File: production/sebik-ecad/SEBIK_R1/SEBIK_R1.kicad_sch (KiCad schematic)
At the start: 87 parts, among them J1 Conn_01x06_Male, J10 Conn_01x02_Male, J11 Conn_01x03_Male, J11 USB_B, J12 Conn_01x02_Male, J13 Conn_01x02_Male, J2 Conn_01x02_Male, J3 Conn_01x02_Male, J4 Conn_01x02_Male, J5 Conn_01x02_Male, J6 Conn_01x02_Male, J7 Conn_01x03_Male, J8 Conn_01x01_Male, J9 Conn_01x01_Male, Q1 2N7002, Q2 2N7002, Q3 2N7002, U1 ATmega328-A, U2 MCP23017_SO, U3 USBLC6-2SC6, U4 FT232RL, U5 MAX31855EASA, U6 MAX31855EASA, U7 MAX31855EASA, U8 LP2985-5.0, Y1 16Mhz

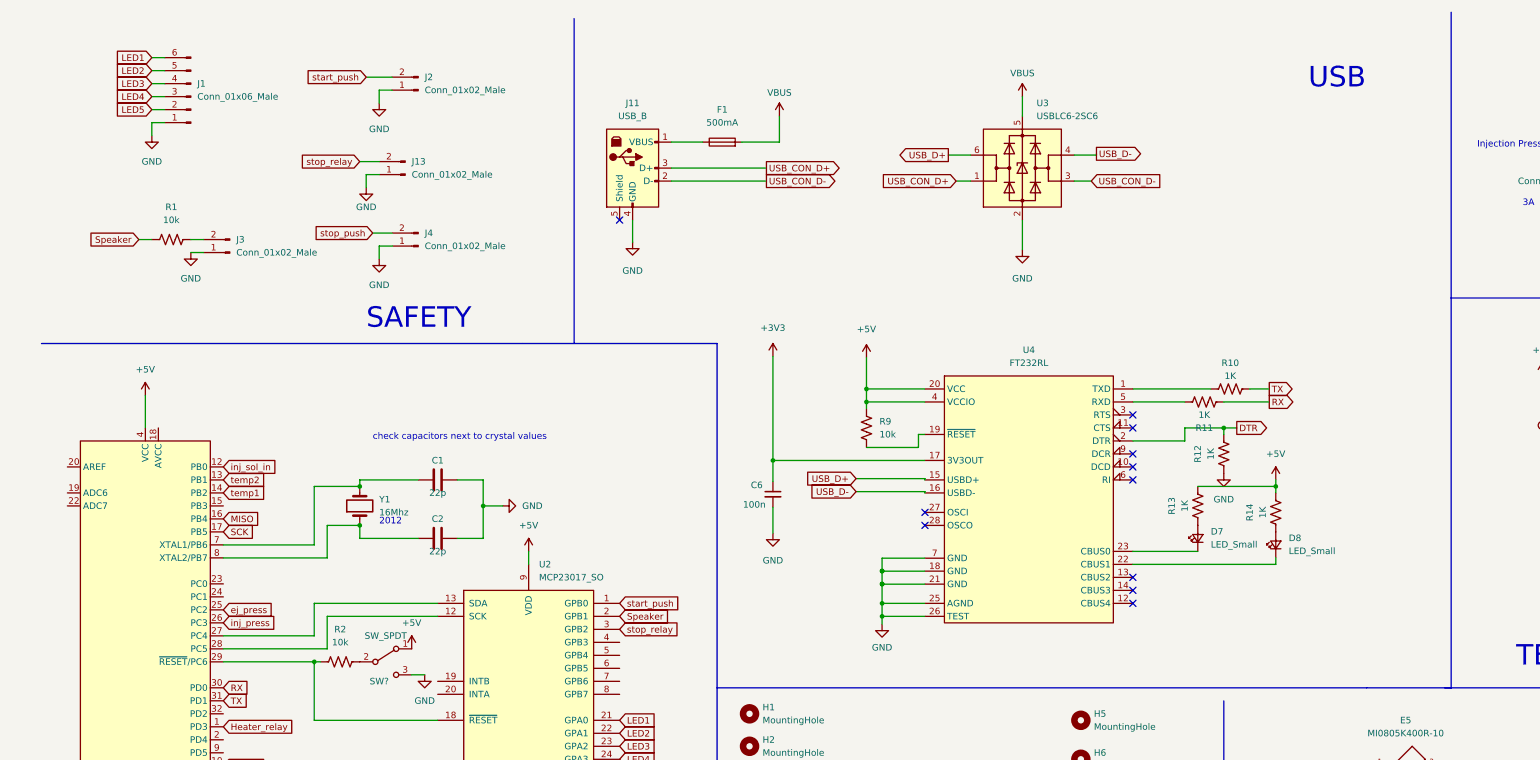
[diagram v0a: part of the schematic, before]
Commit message: Addressed comments from Nick
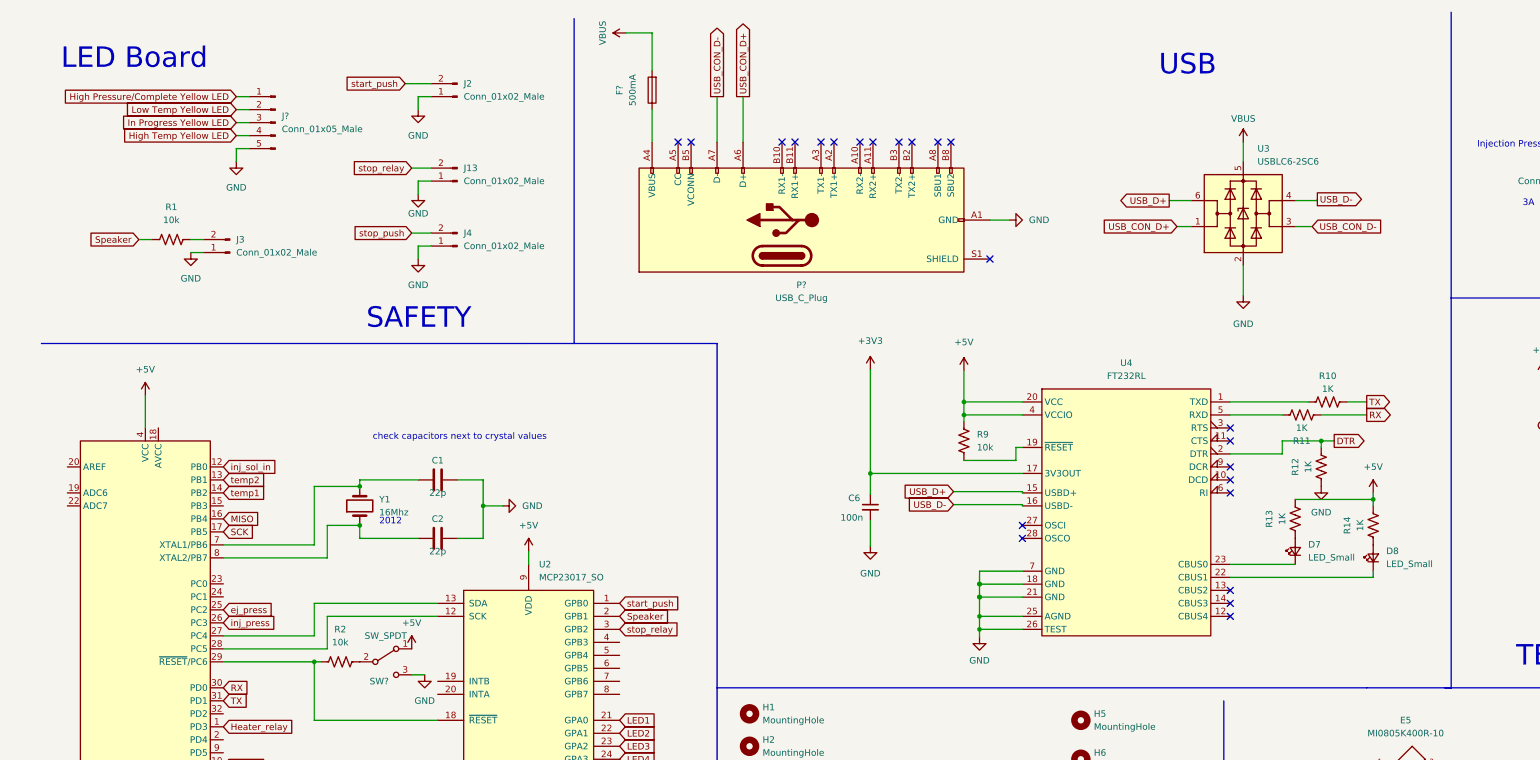
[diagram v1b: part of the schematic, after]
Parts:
- removed F1: 500mA, Fuse:Fuse_1210_3225Metric, symbol Device:Fuse
- removed J1: Conn_01x06_Male, Connector_JST:JST_XH_B6B-XH-AM_1x06_P2.50mm_Vertical, symbol Connector:Conn_01x06_Male
- removed J11: USB_B, Connector_USB:USB_Micro-B_Amphenol_10104110_Horizontal, symbol Connector:USB_B
- added F?: 500mA, Fuse:Fuse_1210_3225Metric, symbol Device:Fuse
- added J?: Conn_01x05_Male, symbol Connector:Conn_01x05_Male
- added P?: USB_C_Plug, symbol Connector:USB_C_Plug
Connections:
- net GND: now also J?.5 (Pin_5), P?.A1 (GND), P?.A12 (GND), P?.B1 (GND), P?.B12 (GND)
- net USB_CON_D+: now also P?.A6 (D+)
- net USB_CON_D-: now also P?.A7 (D-)
- net VBUS: now also F?.2
- new net: F?.1, P?.A4 (VBUS), P?.A9 (VBUS), P?.B4 (VBUS), P?.B9 (VBUS)
- new net High Pressure/Complete Yellow LED: J?.1 (Pin_1)
- new net High Temp Yellow LED: J?.4 (Pin_4)
- new net In Progress Yellow LED: J?.3 (Pin_3)
- new net Low Temp Yellow LED: J?.2 (Pin_2)
- no-connect marks 11 -> 23
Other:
- note added: "LED Board"
- moved on the sheet: C6, D7, D8, J13, J2, J4, R10, R11, R12, R13, R14, R9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
